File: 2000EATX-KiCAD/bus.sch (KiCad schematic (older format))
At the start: 37 parts, among them U302 74LS32, U800 BUSTER, U801 RTC62423, U802 74LS138, U803 74LS08, U804 74LS148

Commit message: Add files via upload
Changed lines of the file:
@@
 $Descr B 17000 11000
 encoding utf-8
-Sheet 7 9
+Sheet 7 10
 Title ""
 Date ""
@@
 	1800 2500 1700 2500
 $Comp
-L Amiga~3000~library:+5V #PWR0224
+L power:+5V #PWR0224
 U 1 1 605A120A
 P 1250 2350
@@
 	1600 5650 1750 5650
 $Comp
-L Amiga~3000~library:+5V #PWR0226
+L power:+5V #PWR0226
 U 1 1 605B0A1C
 P 1750 4450
@@
 	4450 3900 4450 3800
 $Comp
-L Amiga~3000~library:+5V #PWR0227
+L power:+5V #PWR0227
 U 1 1 605C1F0A
 P 4450 3800
@@
 	12750 1900 11900 1900
 $Comp
-L Amiga~3000~library:+5V #PWR0230
+L power:+5V #PWR0230
 U 1 1 605650DB
 P 12800 1750
@@
 $EndComp
 $Comp
-L Amiga~3000~library:GND #PWR0233
+L power:GND #PWR0233
 U 1 1 6062424F
 P 10000 3300
@@
 $EndComp
 $Comp
-L Amiga~3000~library:+5V #PWR0235
+L power:+5V #PWR0235
 U 1 1 60641BA5
 P 13500 1700
@@
 Wire Wire Line
 	13500 2000 13500 1700
-Connection ~ 13500 1700
 Connection ~ 9500 1550
 Wire Wire Line
@@
 	3250 8150 4050 8150
 $Comp
-L Amiga~3000~library:+5V #PWR0238
+L power:+5V #PWR0238
 U 1 1 606958CA
 P 4050 6900
@@
 Wire Wire Line
 	9500 3000 9500 3300
-Connection ~ 10000 3300
 Connection ~ 9500 2000
 Text Notes 13400 9700 2    197  ~ 0
@@
 D3
 $Comp
-L Amiga~3000~library:+5V #PWR0232
+L power:+5V #PWR0232
 U 1 1 605CA78F
 P 9500 1350
@@
 	7650 7450 7650 7250
 $Comp
-L Amiga~3000~library:+5V #PWR0225
+L power:+5V #PWR0225
 U 1 1 605B851F
 P 7650 7250
@@
 	7300 9200 7300 9250
 $Comp
-L Amiga~3000~library:+5V #PWR0241
+L power:+5V #PWR0241
 U 1 1 6060C85C
 P 11000 7150

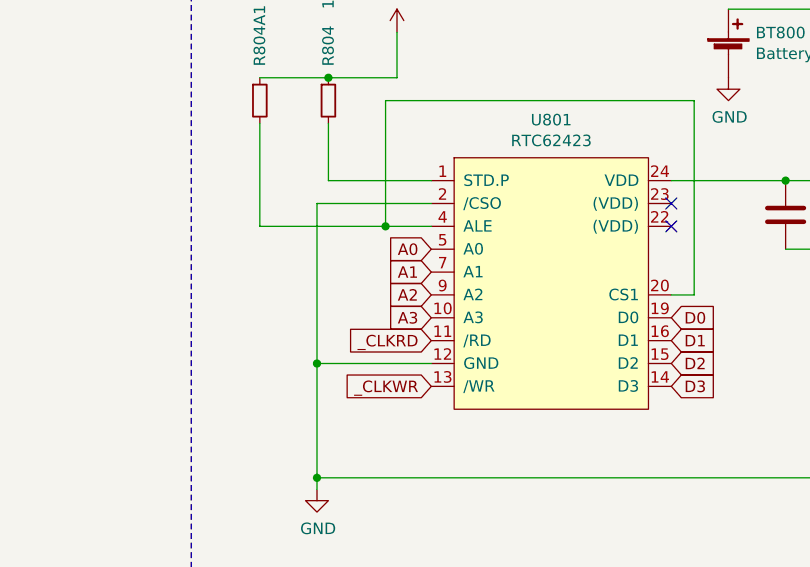
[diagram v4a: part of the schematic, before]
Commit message: Add files via upload
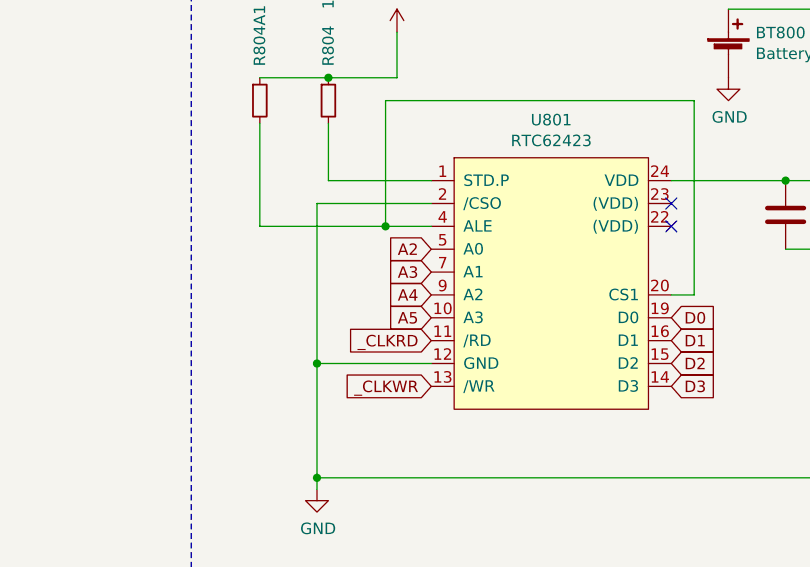
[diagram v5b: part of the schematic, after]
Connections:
- net A0 is gone; now on net A2: U801.5 (A0)
- net A1 is gone; now on net A3: U801.7 (A1)
- net A2: no longer U801.9 (A2)
- net A3: no longer U801.10 (A3)
- new net A4: U801.9 (A2)
- new net A5: U801.10 (A3)
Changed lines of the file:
@@
 	9500 2000 9500 2800
 Text GLabel 7800 8200 0    50   Input ~ 0
-A0
+A2
 Text GLabel 7800 8300 0    50   Input ~ 0
-A1
+A3
 Text GLabel 7800 8400 0    50   Input ~ 0
-A2
+A4
 Text GLabel 7800 8500 0    50   Input ~ 0
-A3
+A5
 Text GLabel 8850 8500 2    50   Input ~ 0
 D0

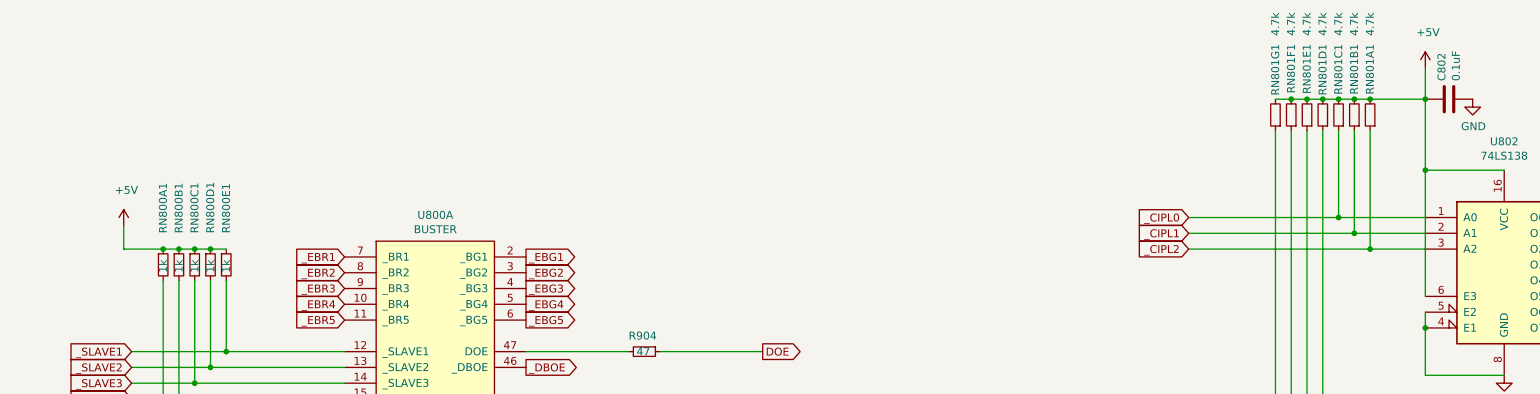
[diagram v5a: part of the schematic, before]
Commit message: Add files via upload
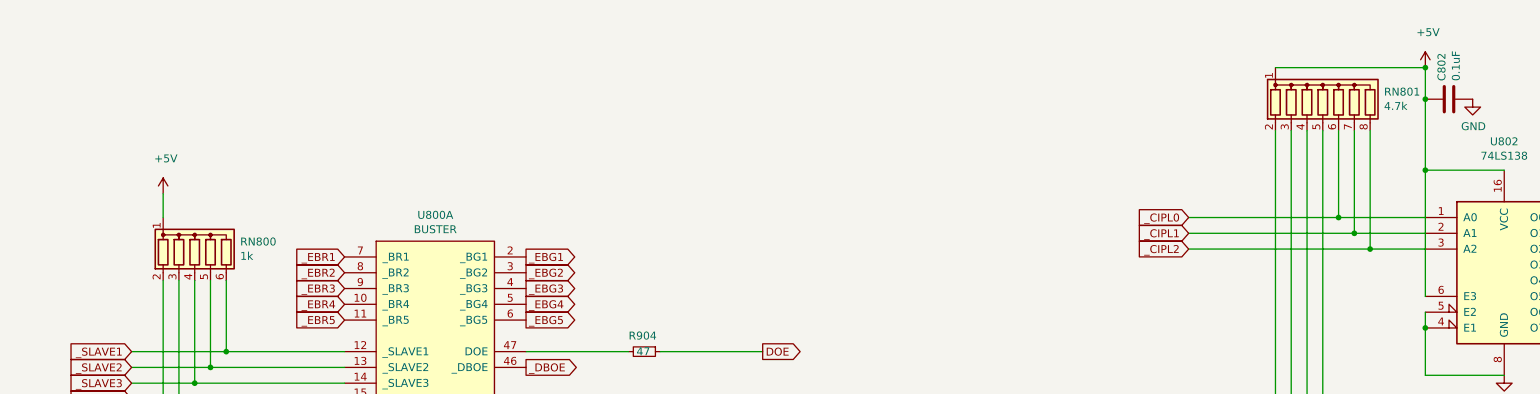
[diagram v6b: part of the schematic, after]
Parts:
- removed RN800A1, RN800B1, RN800C1, RN800D1, RN800E1: 1k, Resistor_SMD:R_1206_3216Metric, symbol Device:R_Small
- removed RN801A1, RN801B1, RN801C1, RN801D1, RN801E1, RN801F1, RN801G1: 4.7k, Resistor_SMD:R_1206_3216Metric, symbol Device:R_Small
- added RN800: 1k, Resistor_THT:R_Array_SIP6, symbol Device:R_Network05
- added RN801: 4.7k, Resistor_THT:R_Array_SIP8, symbol Device:R_Network07
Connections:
- net +5V: now also RN800.1 (common), RN801.1 (common)
- net _CIPL0: now also RN801.6 (R5)
- net _CIPL1: now also RN801.7 (R6)
- net _CIPL2: now also RN801.8 (R7)
- net _EINT1: now also RN801.2 (R1)
- net _EINT4: now also RN801.3 (R2)
- net _EINT5: now also RN801.4 (R3)
- net _EINT7: now also RN801.5 (R4)
- net _SLAVE1: now also RN800.6 (R5)
- net _SLAVE2: now also RN800.5 (R4)
- net _SLAVE3: now also RN800.4 (R3)
- net _SLAVE4: now also RN800.3 (R2)
- net _SLAVE5: now also RN800.2 (R1)
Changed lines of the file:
@@
 Wire Wire Line
 	2650 3550 1500 3550
-$Comp
-L Device:R_Small RN800A1
-U 1 1 6059F77A
-P 1500 2600
-F 0 "RN800A1" V 1500 2800 50  0000 L CNN
-F 1 "1k" V 1500 2550 50  0000 L CNN
-F 2 "Resistor_SMD:R_1206_3216Metric" H 1500 2600 50  0001 C CNN
-F 3 "~" H 1500 2600 50  0001 C CNN
-	1    1500 2600
-	1    0    0    -1
-$EndComp
-$Comp
-L Device:R_Small RN800B1
-U 1 1 605A04B7
-P 1600 2600
-F 0 "RN800B1" V 1600 2800 50  0000 L CNN
-F 1 "1k" V 1600 2550 50  0000 L CNN
-F 2 "Resistor_SMD:R_1206_3216Metric" H 1600 2600 50  0001 C CNN
-F 3 "~" H 1600 2600 50  0001 C CNN
-	1    1600 2600
-	1    0    0    -1
-$EndComp
-$Comp
-L Device:R_Small RN800C1
-U 1 1 605A06F8
-P 1700 2600
-F 0 "RN800C1" V 1700 2800 50  0000 L CNN
-F 1 "1k" V 1700 2550 50  0000 L CNN
-F 2 "Resistor_SMD:R_1206_3216Metric" H 1700 2600 50  0001 C CNN
-F 3 "~" H 1700 2600 50  0001 C CNN
-	1    1700 2600
-	1    0    0    -1
-$EndComp
-$Comp
-L Device:R_Small RN800D1
-U 1 1 605A08C8
-P 1800 2600
-F 0 "RN800D1" V 1800 2800 50  0000 L CNN
-F 1 "1k" V 1800 2550 50  0000 L CNN
-F 2 "Resistor_SMD:R_1206_3216Metric" H 1800 2600 50  0001 C CNN
-F 3 "~" H 1800 2600 50  0001 C CNN
-	1    1800 2600
-	1    0    0    -1
-$EndComp
-$Comp
-L Device:R_Small RN800E1
-U 1 1 605A0A47
-P 1900 2600
-F 0 "RN800E1" V 1900 2800 50  0000 L CNN
-F 1 "1k" V 1900 2550 50  0000 L CNN
-F 2 "Resistor_SMD:R_1206_3216Metric" H 1900 2600 50  0001 C CNN
-F 3 "~" H 1900 2600 50  0001 C CNN
-	1    1900 2600
-	1    0    0    -1
-$EndComp
-Wire Wire Line
-	1900 2500 1800 2500
-Wire Wire Line
-	1250 2500 1250 2350
-Connection ~ 1500 2500
-Wire Wire Line
-	1500 2500 1250 2500
-Connection ~ 1600 2500
-Wire Wire Line
-	1600 2500 1500 2500
-Connection ~ 1700 2500
-Wire Wire Line
-	1700 2500 1600 2500
-Connection ~ 1800 2500
-Wire Wire Line
-	1800 2500 1700 2500
+Wire Wire Line
+	1500 2300 1500 2150
 $Comp
 L power:+5V #PWR0224
 U 1 1 605A120A
-P 1250 2350
-F 0 "#PWR0224" H 1250 2200 50  0001 C CNN
-F 1 "+5V" H 1267 2573 50  0000 C CNN
-F 2 "" H 1250 2350 50  0001 C CNN
-F 3 "" H 1250 2350 50  0001 C CNN
-	1    1250 2350
+P 1500 2150
+F 0 "#PWR0224" H 1500 2000 50  0001 C CNN
+F 1 "+5V" H 1517 2373 50  0000 C CNN
+F 2 "" H 1500 2150 50  0001 C CNN
+F 3 "" H 1500 2150 50  0001 C CNN
+	1    1500 2150
 	1    0    0    -1
 $EndComp
@@
 	1    0    0    -1
 $EndComp
-Connection ~ 8850 1550
-$Comp
-L Device:R_Small RN801D1
-U 1 1 6056B172
-P 8850 1650
-F 0 "RN801D1" V 8850 1200 50  0000 L CNN
-F 1 "4.7k" V 8850 1000 50  0000 L CNN
-F 2 "Resistor_SMD:R_1206_3216Metric" H 8850 1650 50  0001 C CNN
-F 3 "~" H 8850 1650 50  0001 C CNN
-	1    8850 1650
-	-1   0    0    1
-$EndComp
-Connection ~ 9050 1550
-$Comp
-L Device:R_Small RN801B1
-U 1 1 6056AA7A
-P 9050 1650
-F 0 "RN801B1" V 9050 1200 50  0000 L CNN
-F 1 "4.7k" V 9050 1000 50  0000 L CNN
-F 2 "Resistor_SMD:R_1206_3216Metric" H 9050 1650 50  0001 C CNN
-F 3 "~" H 9050 1650 50  0001 C CNN
-	1    9050 1650
-	-1   0    0    1
-$EndComp
-$Comp
-L Device:R_Small RN801G1
-U 1 1 6056BC64
-P 8550 1650
-F 0 "RN801G1" V 8550 1200 50  0000 L CNN
-F 1 "4.7k" V 8550 1000 50  0000 L CNN
-F 2 "Resistor_SMD:R_1206_3216Metric" H 8550 1650 50  0001 C CNN
-F 3 "~" H 8550 1650 50  0001 C CNN
-	1    8550 1650
-	-1   0    0    1
-$EndComp
-Wire Wire Line
-	8550 1550 8650 1550
-Connection ~ 8650 1550
-$Comp
-L Device:R_Small RN801F1
-U 1 1 6056B8F7
-P 8650 1650
-F 0 "RN801F1" V 8650 1200 50  0000 L CNN
-F 1 "4.7k" V 8650 1000 50  0000 L CNN
-F 2 "Resistor_SMD:R_1206_3216Metric" H 8650 1650 50  0001 C CNN
-F 3 "~" H 8650 1650 50  0001 C CNN
-	1    8650 1650
-	-1   0    0    1
-$EndComp
-Wire Wire Line
-	8750 1550 8850 1550
-Wire Wire Line
-	8650 1550 8750 1550
-Connection ~ 8750 1550
-$Comp
-L Device:R_Small RN801E1
-U 1 1 6056B568
-P 8750 1650
-F 0 "RN801E1" V 8750 1200 50  0000 L CNN
-F 1 "4.7k" V 8750 1000 50  0000 L CNN
-F 2 "Resistor_SMD:R_1206_3216Metric" H 8750 1650 50  0001 C CNN
-F 3 "~" H 8750 1650 50  0001 C CNN
-	1    8750 1650
-	-1   0    0    1
-$EndComp
-Wire Wire Line
-	8850 1550 8950 1550
-Wire Wire Line
-	8950 1550 9050 1550
-Connection ~ 8950 1550
-$Comp
-L Device:R_Small RN801C1
-U 1 1 6056AE33
-P 8950 1650
-F 0 "RN801C1" V 8950 1200 50  0000 L CNN
-F 1 "4.7k" V 8950 1000 50  0000 L CNN
-F 2 "Resistor_SMD:R_1206_3216Metric" H 8950 1650 50  0001 C CNN
-F 3 "~" H 8950 1650 50  0001 C CNN
-	1    8950 1650
-	-1   0    0    1
-$EndComp
-Wire Wire Line
-	9050 1550 9150 1550
-Wire Wire Line
-	9150 1550 9500 1550
-Connection ~ 9150 1550
-$Comp
-L Device:R_Small RN801A1
-U 1 1 605615E6
-P 9150 1650
-F 0 "RN801A1" V 9150 1200 50  0000 L CNN
-F 1 "4.7k" V 9150 1000 50  0000 L CNN
-F 2 "Resistor_SMD:R_1206_3216Metric" H 9150 1650 50  0001 C CNN
-F 3 "~" H 9150 1650 50  0001 C CNN
-	1    9150 1650
-	-1   0    0    1
-$EndComp
 $Comp
 L Device:R_Small R804
@@
 	1    0    0    -1
 $EndComp
+$Comp
+L Device:R_Network07 RN801
+U 1 1 6113DD54
+P 8850 1550
+F 0 "RN801" H 9238 1596 50  0000 L CNN
+F 1 "4.7k" H 9238 1505 50  0000 L CNN
+F 2 "Resistor_THT:R_Array_SIP8" V 9325 1550 50  0001 C CNN
+F 3 "http://www.vishay.com/docs/31509/csc.pdf" H 8850 1550 50  0001 C CNN
+	1    8850 1550
+	1    0    0    -1
+$EndComp
+Wire Wire Line
+	9500 1350 8550 1350
+Connection ~ 9500 1350
+$Comp
+L Device:R_Network05 RN800
+U 1 1 61163DED
+P 1700 2500
+F 0 "RN800" H 1988 2546 50  0000 L CNN
+F 1 "1k" H 1988 2455 50  0000 L CNN
+F 2 "Resistor_THT:R_Array_SIP6" V 2075 2500 50  0001 C CNN
+F 3 "http://www.vishay.com/docs/31509/csc.pdf" H 1700 2500 50  0001 C CNN
+	1    1700 2500
+	1    0    0    -1
+$EndComp

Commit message: Add files via upload
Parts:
- U801: footprint Package_SO:SOIC-24W_7.5x15.4mm_P1.27mm -> Package_SO:SOP-24_7.5x15.4mm_P1.27mm
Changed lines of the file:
@@
 F 0 "U801" H 8325 9065 50  0000 C CNN
 F 1 "RTC62423" H 8325 8974 50  0000 C CNN
-F 2 "Package_SO:SOIC-24W_7.5x15.4mm_P1.27mm" H 8150 8600 50  0001 C CNN
+F 2 "Package_SO:SOP-24_7.5x15.4mm_P1.27mm" H 8150 8600 50  0001 C CNN
 F 3 "" H 8150 8600 50  0001 C CNN
 	1    8350 8350
